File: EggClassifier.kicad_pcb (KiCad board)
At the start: 2 copper layers, 140 x 80 mm, 78 parts, among them J1 ST-LINK, J10 LCD_CHAR, J11 SERVO2, J12 BME280, J13 UART1, J14 FAN, J15 UART2, J16 AS7265X, J17 TFT_SPI, J18 SD_CARD, J2 USB_A, J3 Jumper, J5 POWER, J6 DCMI_CAMERA, J7 USER_GPIO, J8 SERVO1, J9 ADC_IN, Q1 BCP56, Q2 BCP56, Q3 BCP56, SW1 RESET SW, U1 LM2676S-5, U2 AMS1117-3.3, U3 STM32H743VITx, U4 W25Q128, Y1 25MHZ

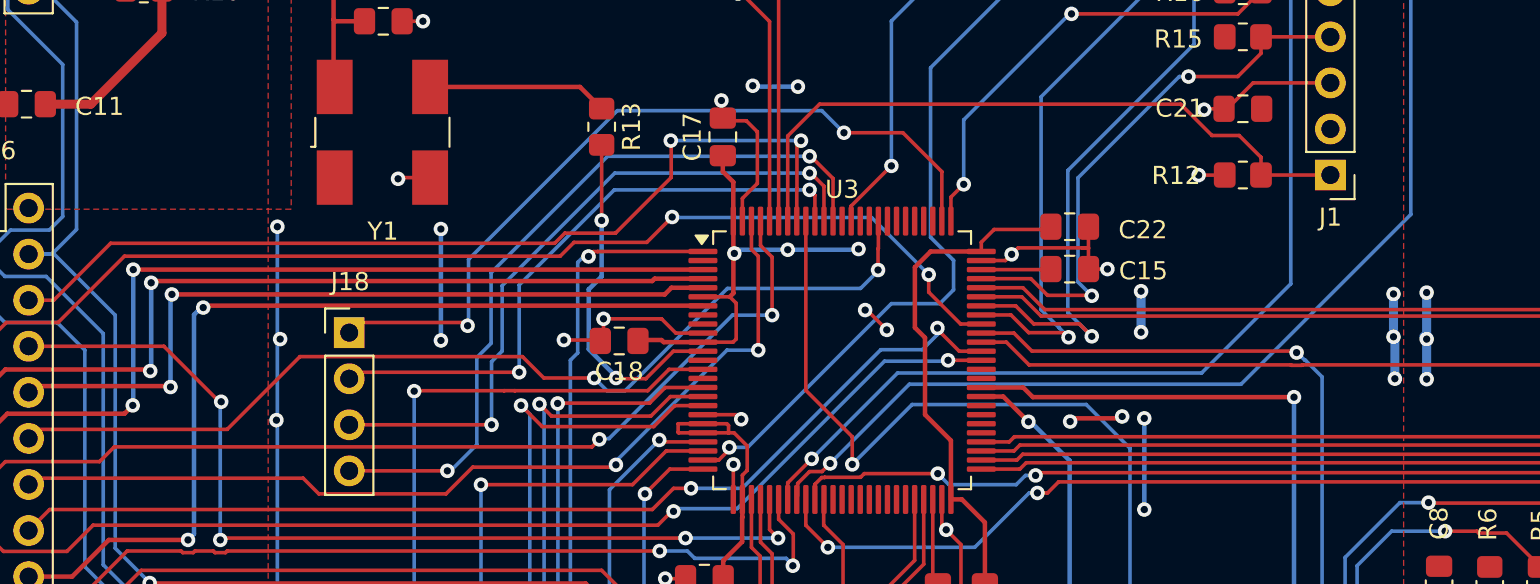
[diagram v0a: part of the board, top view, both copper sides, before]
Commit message: final version of 80mmx140mm PCB
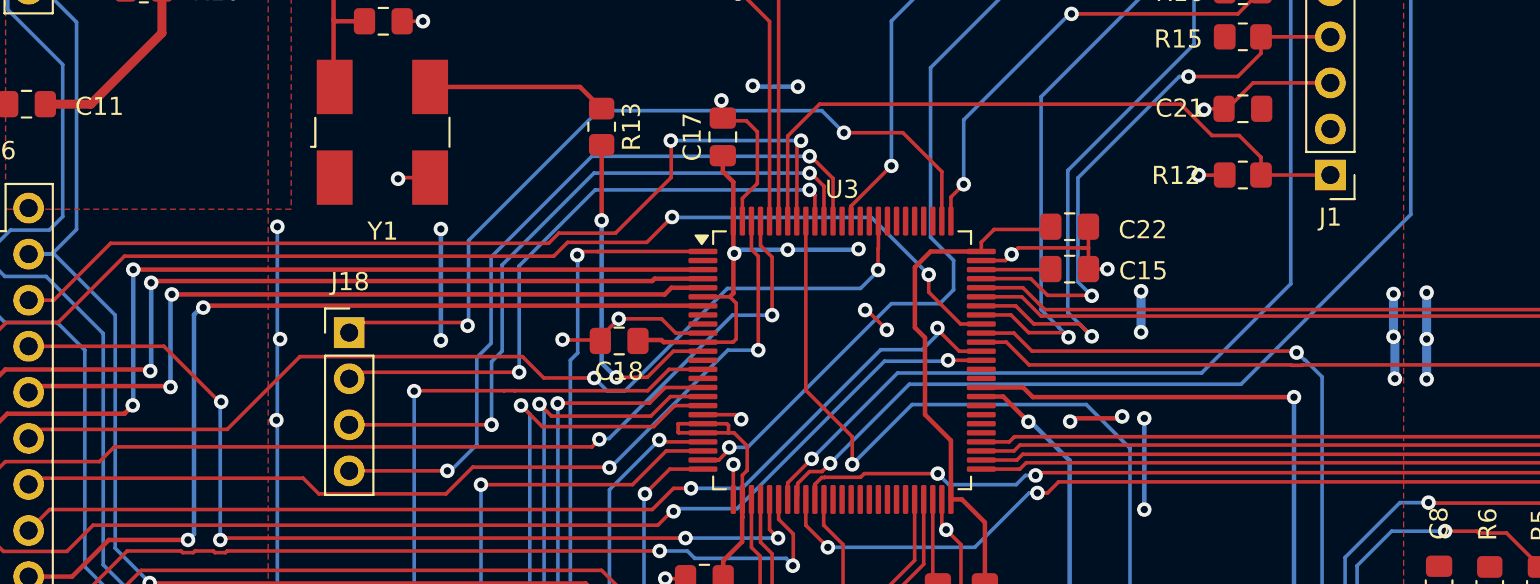
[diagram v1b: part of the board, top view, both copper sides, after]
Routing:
- net GND: track 133.5 -> 132.7 mm
- net Net-(U3-PH0): track 19.2 -> 18.5 mm
- net SPI1_MISO: track 38.3 -> 39.0 mm
- net SPI1_MOSI: track 33.9 -> 34.5 mm
- net SPI1_SCK: track 41.8 -> 42.3 mm
